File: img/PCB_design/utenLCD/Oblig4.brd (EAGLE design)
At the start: 155.9 x 114.3 mm, 7 parts

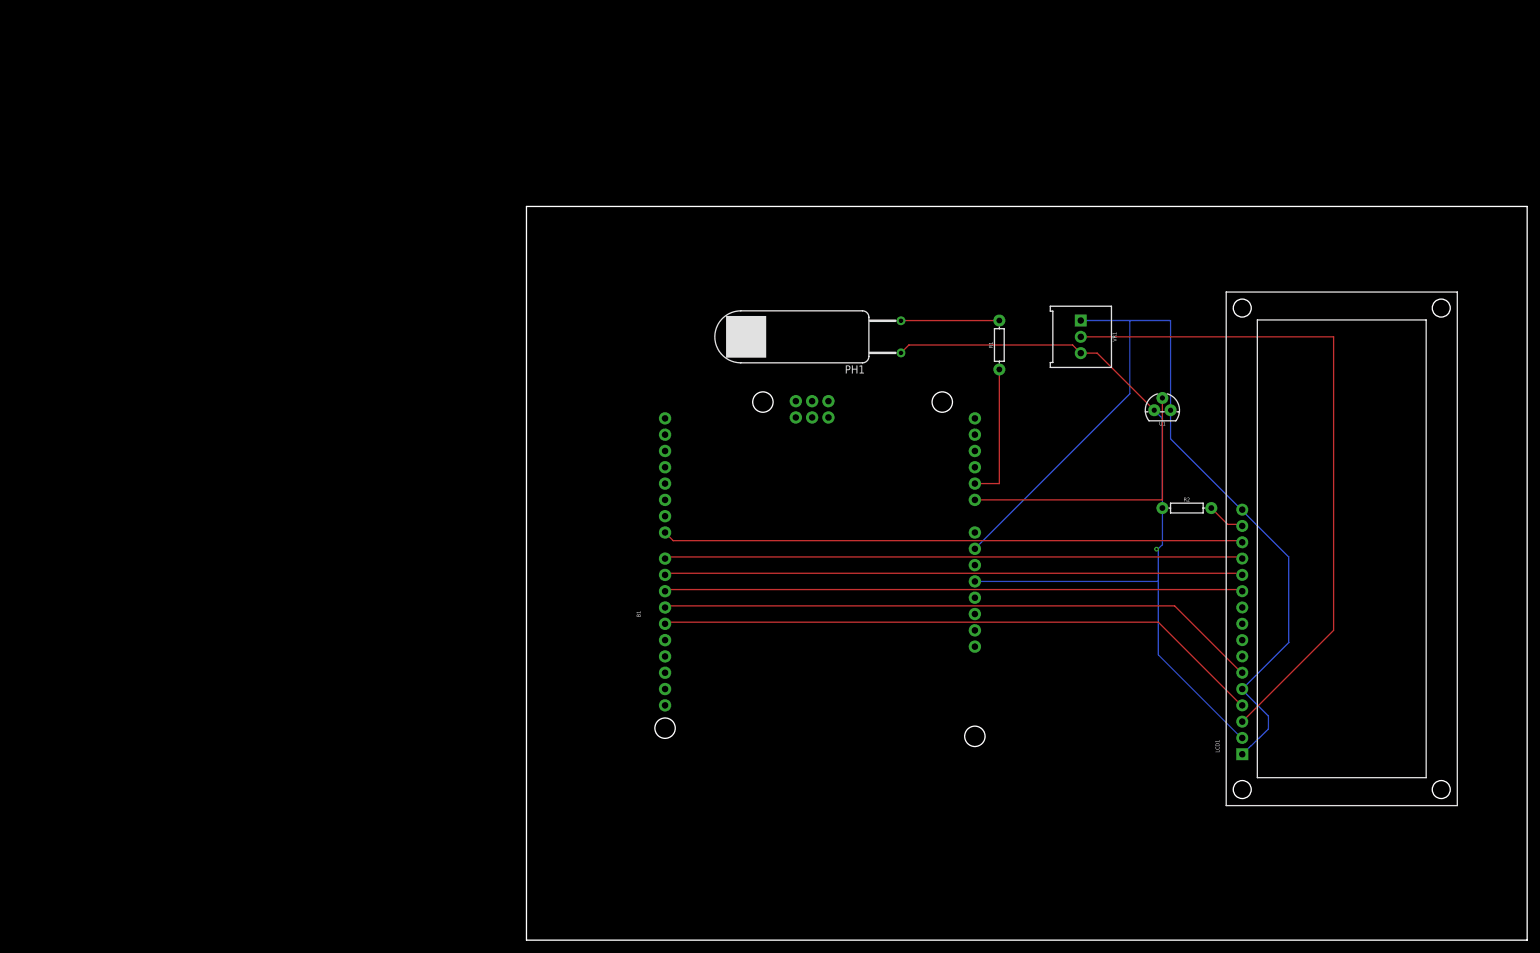
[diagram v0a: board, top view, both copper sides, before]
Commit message: Oppdatert
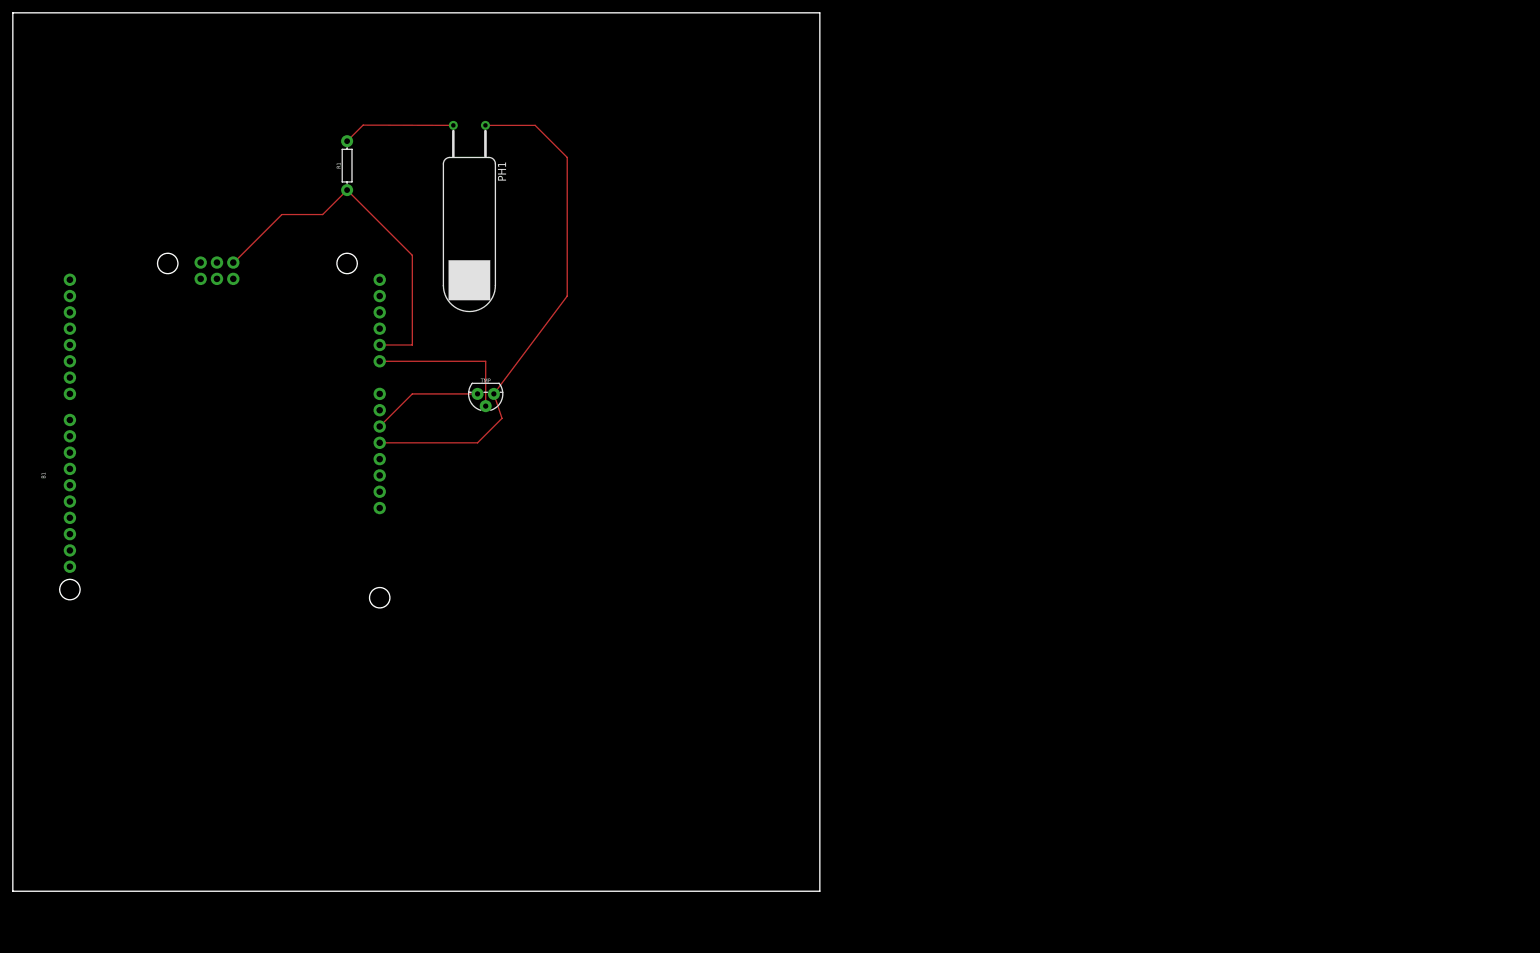
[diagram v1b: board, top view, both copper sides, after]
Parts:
- removed LCD1: LCD-16X2SILK, SparkFun-Displays:LCD-16X2
- removed R2: 220 OHM, SparkFun-Resistors:AXIAL-0.3
- removed U1: (no value), SparkFun-Sensors:TO-92
- removed VR1: 10k, SparkFun-Resistors:TRIMPOT-PTH-3386U
- added TMP: (no value), SparkFun-Sensors:TO-92
- R1: value 10K OHM -> 220 OHM
- moved R1 105.4 mm to (-47.0, 110.5)
- moved B1 95.2 mm to (-66.0, 62.2)
- moved PH1 68.2 mm to (-27.9, 111.8), turned to 180 degrees
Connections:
- removed net N$1 (its old number): B1.A1, R1.P$1
- removed net N$10: B1.D11, LCD1.6
- removed net N$11: B1.D9, LCD1.12
- removed net N$12: B1.D8, LCD1.13
- removed net N$13: B1.D10, LCD1.11
- removed net N$2: B1.A0, U1.2
- removed net N$3: B1.5V, LCD1.2, PH1.1, R2.P$1, U1.1, VR1.3
- removed net N$6: LCD1.3, VR1.2
- removed net N$7: LCD1.15, R2.P$2
- removed net N$8: B1.D7, LCD1.14
- removed net N$9: B1.D12, LCD1.4
- new net S$1: B1.A1, B1.GND@4, R1.P$1
- new net S$2: B1.A0, TMP.2
- new net S$3: B1.GND@1, TMP.3
- net N$4: now also B1.5V, PH1.1, TMP.1; no longer B1.GND@2, LCD1.1, LCD1.16, LCD1.5, U1.3, VR1.1
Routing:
- net N$3: track 130.7 -> 0.00 mm, vias 1 -> 0
- net N$6: track 105.8 -> 0.00 mm
- net N$9: track 95.5 -> 0.00 mm
- net N$10: track 94.4 -> 0.00 mm
- net N$8: track 90.5 -> 0.00 mm
- net N$13: track 90.2 -> 0.00 mm
- net N$11: track 90.2 -> 0.00 mm
- net N$12: track 90.2 -> 0.00 mm
- net N$4: track 141.6 -> 80.1 mm
- net S$1: track 0.00 -> 55.9 mm
- net N$2: track 45.1 -> 0.00 mm
- net S$2: track 0.00 -> 23.5 mm
- net N$1 (its old number): track 21.6 -> 0.00 mm
- net S$3: track 0.00 -> 17.3 mm
- net N$7: track 5.95 -> 0.00 mm
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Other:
- board size 155.9 x 114.3 mm -> 125.7 x 136.8 mm
